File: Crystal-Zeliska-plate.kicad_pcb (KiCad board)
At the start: 2 copper layers, 182.6 x 114.3 mm, 0 parts

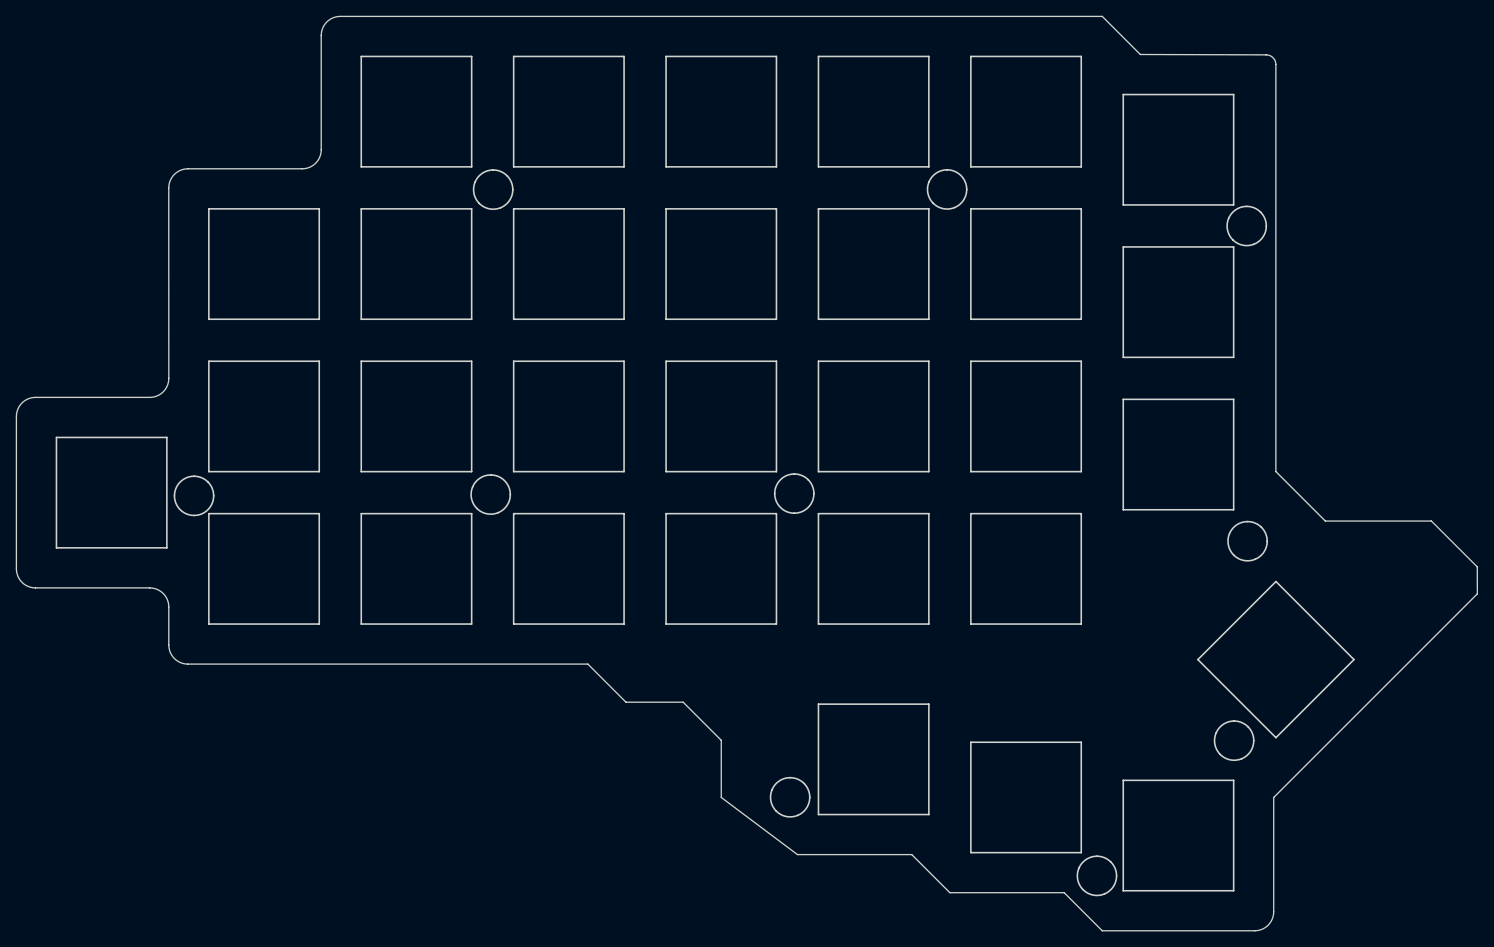
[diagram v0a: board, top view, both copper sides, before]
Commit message: updated Gerber
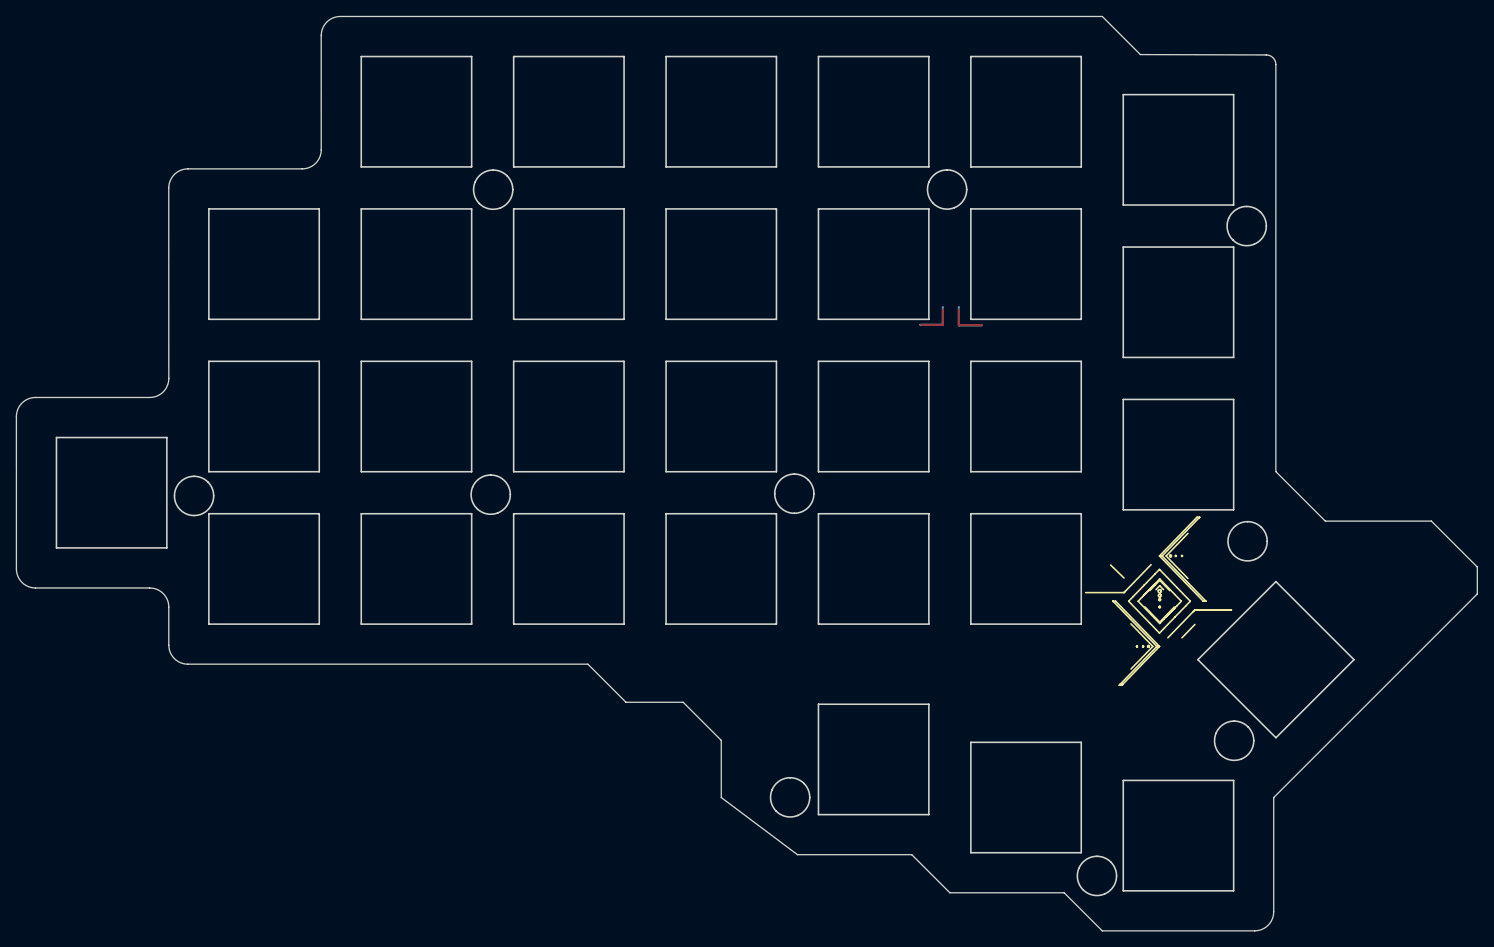
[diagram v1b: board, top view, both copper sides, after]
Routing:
- net (no net): track 0.00 -> 19.8 mm
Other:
- outline, holes or cut-outs redrawn
